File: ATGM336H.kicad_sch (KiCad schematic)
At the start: 8 parts, among them IC1 ATGM336H-5N31, U9 M24C32

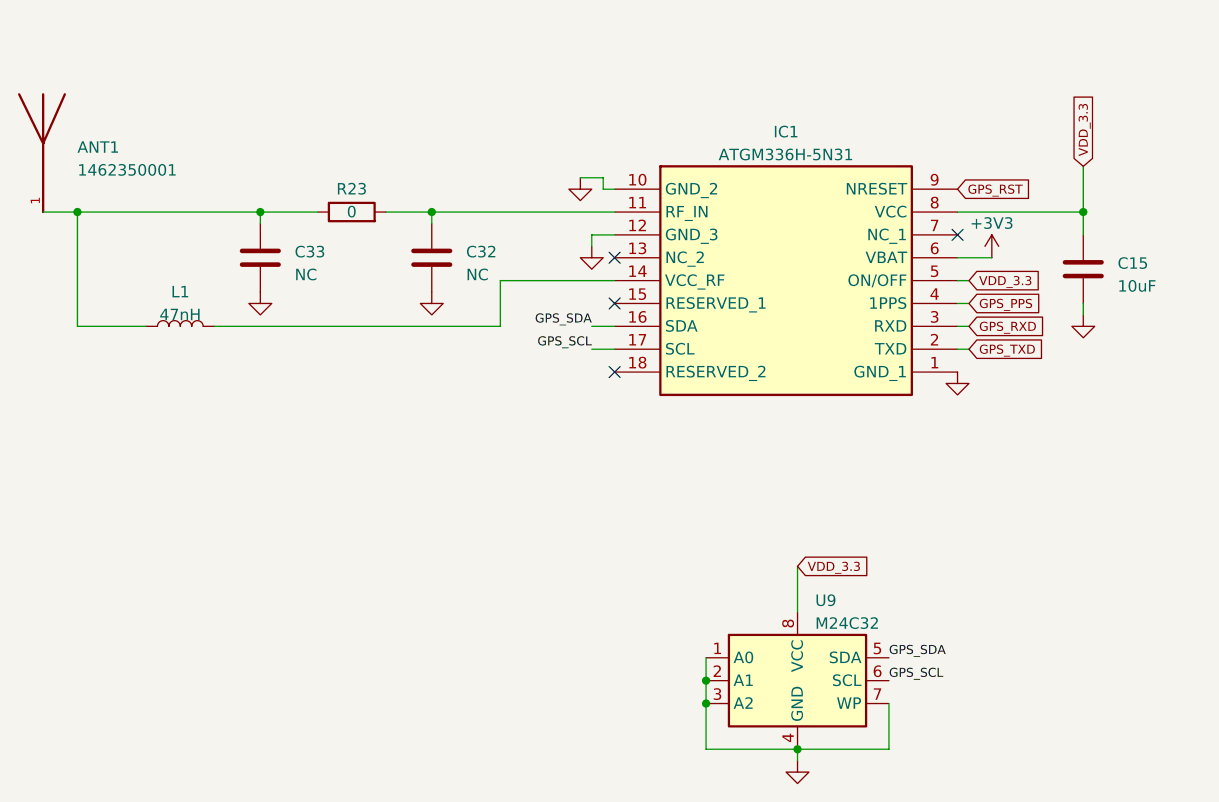
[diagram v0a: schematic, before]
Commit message: bottom board conn. done
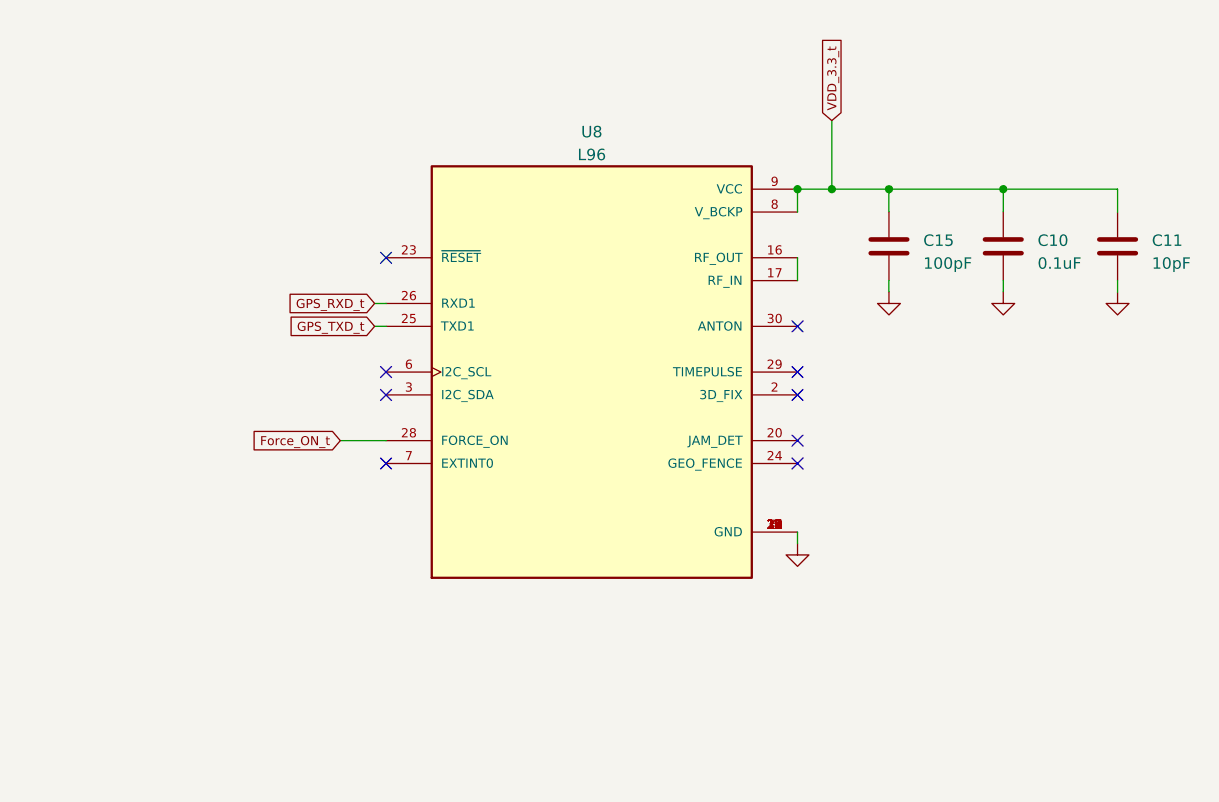
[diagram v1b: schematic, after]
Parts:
- removed ANT1: 1462350001, Molex GPS antenna:ANT_1462350001, symbol 1462350001:1462350001
- removed C32, C33: NC, Capacitor_SMD:C_0402_1005Metric_Pad0.74x0.62mm_HandSolder, symbol Device:C
- removed IC1: ATGM336H-5N31, ATGM336H-5N31:ATGM336H5N31, symbol ATGM336H-5N31:ATGM336H-5N31
- removed L1: 47nH, Inductor_SMD:L_0402_1005Metric, symbol Device:L
- removed R23: 0, Resistor_SMD:R_0402_1005Metric_Pad0.72x0.64mm_HandSolder, symbol Device:R
- removed U9: M24C32, Package_SO:TSSOP-8_4.4x3mm_P0.65mm, symbol Memory_EEPROM:24LC32
- added C10: 0.1uF, Capacitor_SMD:C_0402_1005Metric_Pad0.74x0.62mm_HandSolder, symbol Device:C
- added C11: 10pF, Capacitor_SMD:C_0402_1005Metric_Pad0.74x0.62mm_HandSolder, symbol Device:C
- added U8: L96, L96 (1):XCVR_L96, symbol L96:L96
- C15: value 10uF -> 100pF
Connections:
- net GND: now also C10.2, C11.2, U8.10 (GND), U8.11 (GND), U8.12 (GND), U8.13 (GND), U8.14 (GND), U8.15 (GND), U8.18 (GND), U8.19 (GND), U8.21 (GND), U8.22 (GND), U8.27 (GND), U8.31 (GND), U8.4 (GND), U8.5 (GND)
- net VDD_3.3 renamed VDD_3.3_t
- net VDD_3.3_t: now also C10.1, C11.1, U8.8 (V_BCKP), U8.9 (VCC)
- new net: U8.16 (RF_OUT), U8.17 (RF_IN)
- new net Force_ON_t: U8.28 (FORCE_ON)
- new net GPS_RXD_t: U8.26 (RXD1)
- new net GPS_TXD_t: U8.25 (TXD1)
- no-connect marks 4 -> 9
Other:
- moved on the sheet: C15
